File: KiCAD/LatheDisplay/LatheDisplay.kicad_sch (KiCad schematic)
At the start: 44 parts, among them J1 Screw_Terminal_01x02, J2 Screw_Terminal_01x03, J3 AVR-ISP-6, J4 Conn_01x06_Pin, U1 D168K, U10 LM4040DBZ-4.1, U11 LM7812_TO220, U12 LM7912_TO220, U13 LM7805_TO220, U14 IC_Socket, U15 IC_Socket, U16 IC_Socket, U17 IC_Socket, U18 IC_Socket, U2 D168K, U3 D168K, U4 D168K, U5 D168K, U6 ICM7218B, U7 ATmega328-P, U8 TLC3541, U9 INA121

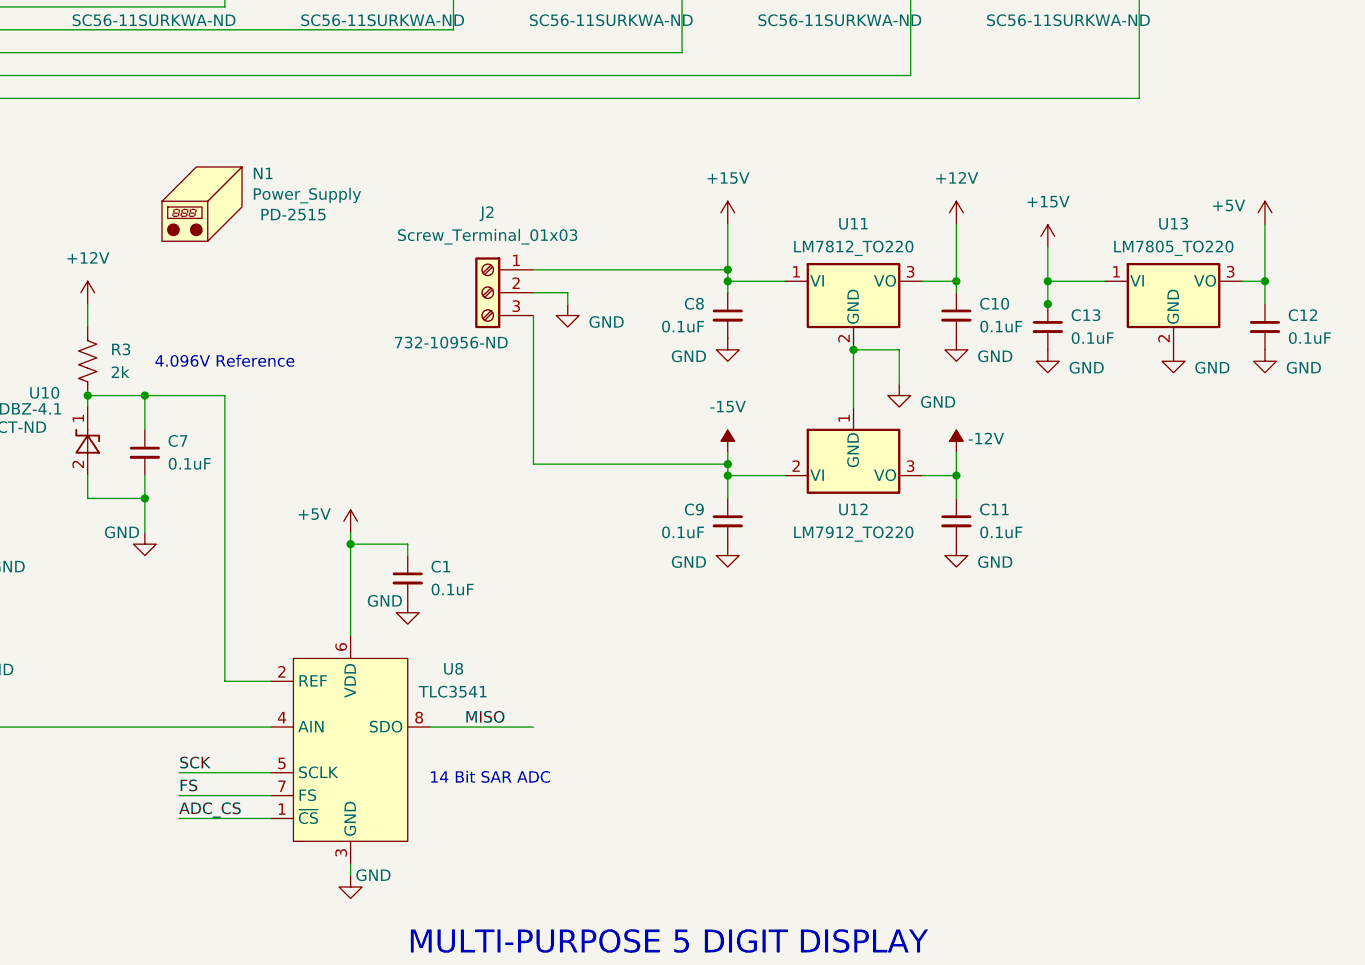
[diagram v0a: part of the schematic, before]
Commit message: save lathe stuff
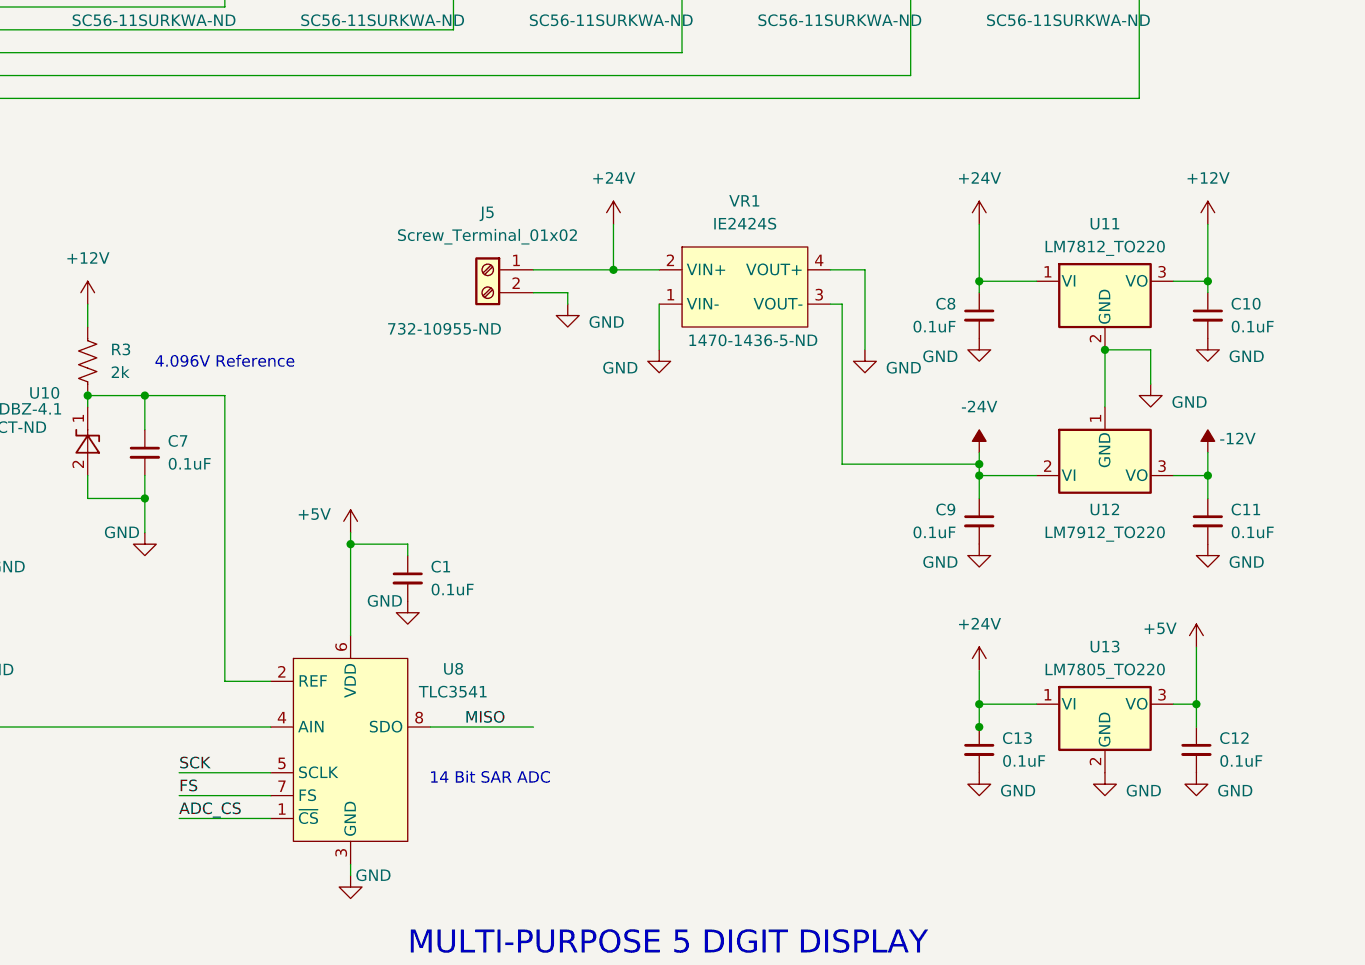
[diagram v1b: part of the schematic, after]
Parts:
- removed J2: Screw_Terminal_01x03, models:3-pin-terminal, symbol Connector:Screw_Terminal_01x03
- removed N1: Power_Supply, symbol Mechanical:Housing
- added J5: Screw_Terminal_01x02, models:691137710002, symbol Connector:Screw_Terminal_01x02
- added VR1: IE2424S, symbol my_DCDC:IE2424S
- J4: footprint Connector_PinHeader_2.54mm:PinHeader_1x06_P2.54mm_Horizontal -> Connector_PinHeader_2.54mm:PinHeader_1x06_P2.54mm_Vertical
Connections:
- net GND: now also J5.2 (Pin_2), VR1.1 (VIN-), VR1.4 (VOUT+)
- net +15V: no longer names the net of C13.1, U13.1 (VI)
- net +15V: no longer C8.1, U11.1 (VI)
- net -15V renamed -24V
- net -24V: now also VR1.3 (VOUT-)
- new net +24V: C8.1, J5.1 (Pin_1), U11.1 (VI), VR1.2 (VIN+)
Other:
- moved on the sheet: C10, C11, C12, C13, C8, C9, U11, U12, U13
